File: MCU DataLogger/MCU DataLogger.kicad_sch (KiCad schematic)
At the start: 25 parts, among them U1 24LC1025, U2 DS1337S_, U3 ATMEGA328P-AN, U4 24LC1025, Y1 32.768 KHz, Y2 16MHz

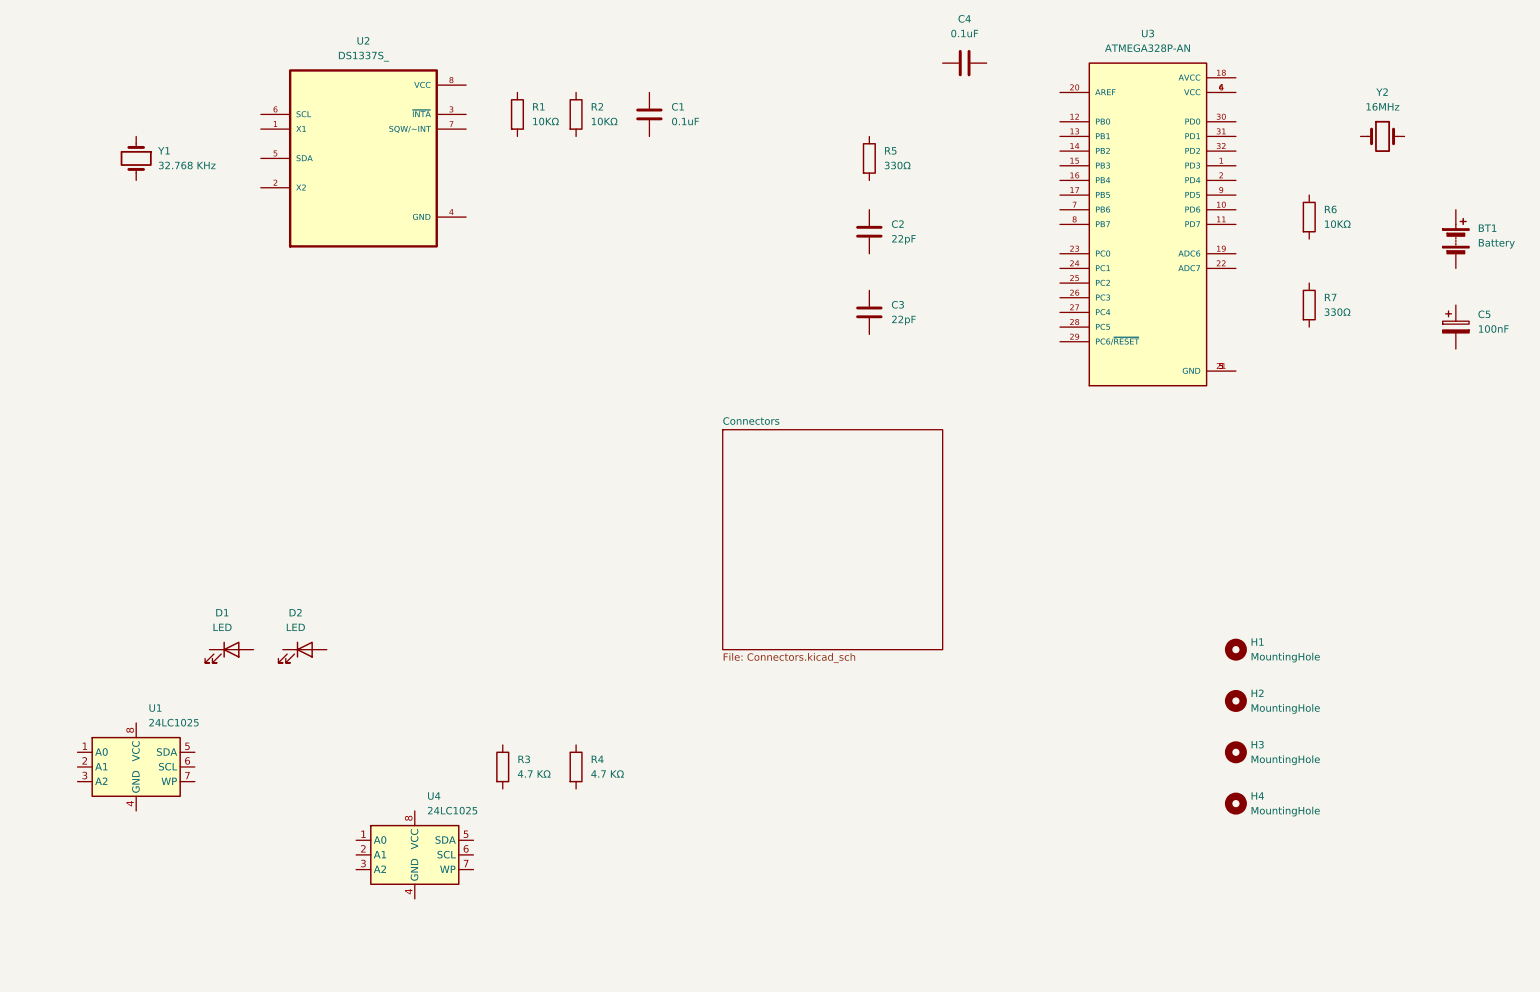
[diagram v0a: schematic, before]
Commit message: MCU Datalogger Project Schematic Complete
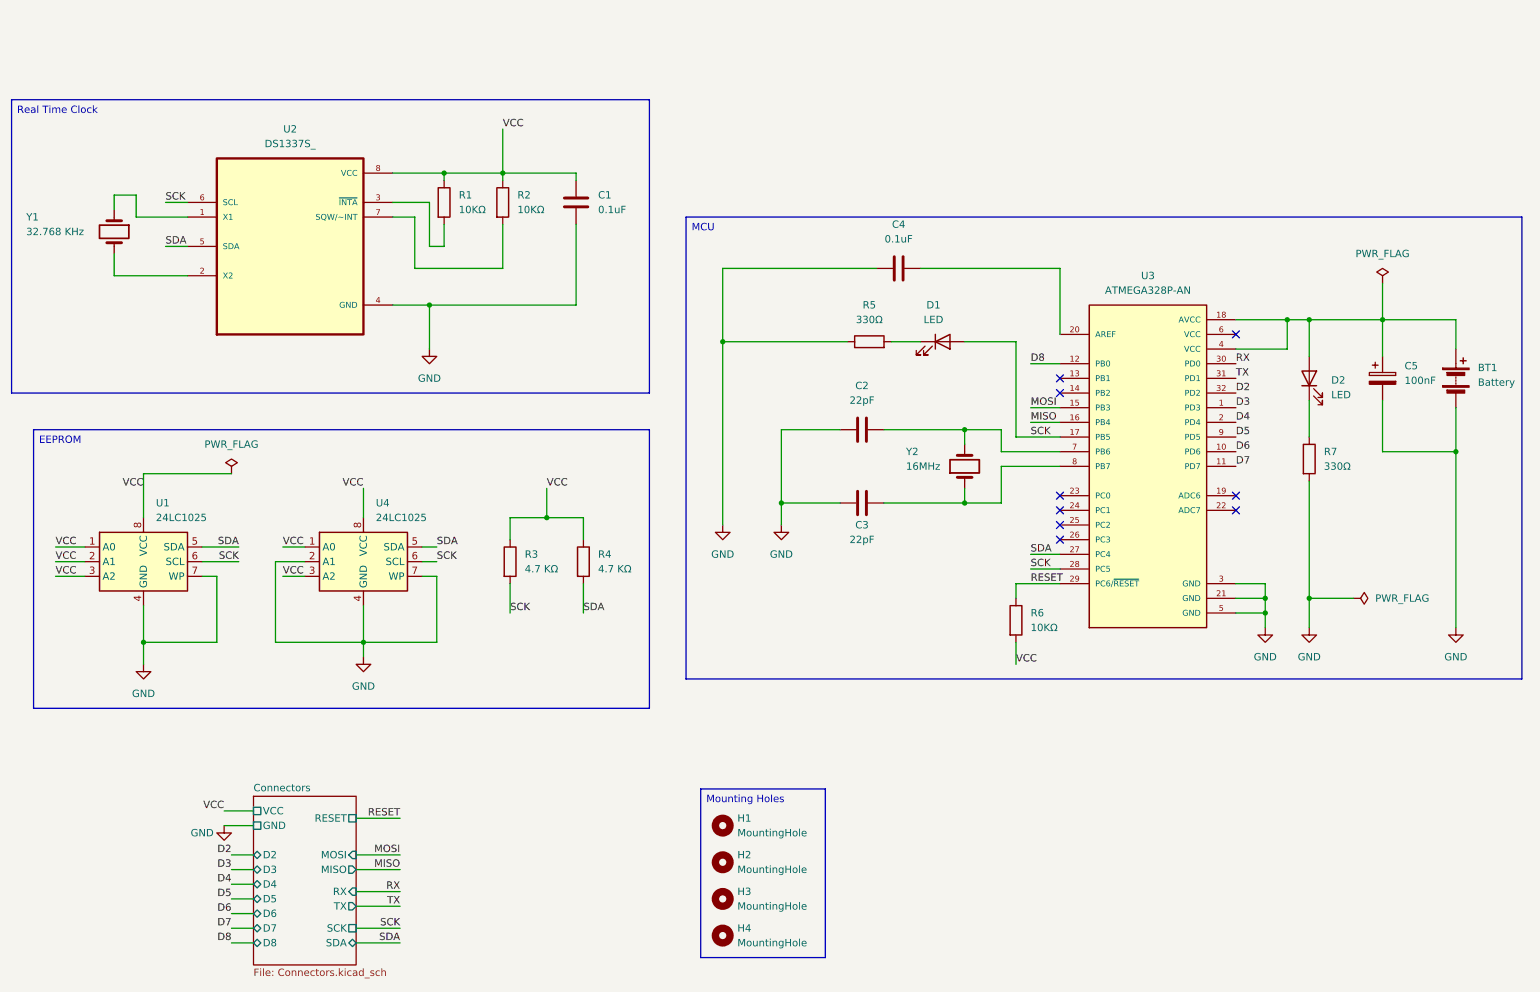
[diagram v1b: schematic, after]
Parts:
- U3: footprint ATMEGA328P:QFP80P900X900X120-32N -> ATMEGA328P-AN:QFP80P900X900X120-32N
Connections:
- net VCC: now reaches C1.1
- net VCC: now also R1.1, R2.1, R3.1, R4.1, R6.2, U1.1 (A0), U1.2 (A1), U1.3 (A2), U1.8 (VCC), U2.8 (VCC), U4.1 (A0), U4.3 (A2), U4.8 (VCC)
- net GND: now reaches C1.2
- net GND: now also BT1.2 (-), C2.1, C3.1, C4.1, C5.2, R5.1, R7.2, U1.4 (GND), U1.7 (WP), U2.4 (GND), U3.21 (GND), U3.3 (GND), U3.5 (GND), U4.2 (A1), U4.4 (GND), U4.7 (WP)
- net D3: now reaches U3.1 (PD3)
- net D6: now reaches U3.10 (PD6)
- net D7: now reaches U3.11 (PD7)
- net D8: now reaches U3.12 (PB0)
- net MOSI: now reaches U3.15 (PB3)
- net MISO: now reaches U3.16 (PB4)
- net SCK: now reaches U3.17 (PB5)
- net SCK: now also D1.2 (A), R3.2, U1.6 (SCL), U2.6 (SCL), U3.28 (PC5), U4.6 (SCL)
- net at U3.18 (AVCC): now also BT1.1 (+), C5.1, D2.2 (A), U3.4 (VCC)
- net D4: now reaches U3.2 (PD4)
- net at U3.20 (AREF): now also C4.2
- net SDA: now reaches U3.27 (PC4)
- net SDA: now also R4.2, U1.5 (SDA), U2.5 (SDA), U4.5 (SDA)
- net RESET: now reaches U3.29 (PC6/~{RESET})
- net RESET: now also R6.1
- net RX: now reaches U3.30 (PD0)
- net TX: now reaches U3.31 (PD1)
- net D2: now reaches U3.32 (PD2)
- net at U3.6 (VCC): no longer U3.4 (VCC)
- net at U3.7 (PB6): now also C2.2, Y2.2
- net at U3.8 (PB7): now also C3.2, Y2.1
- net D5: now reaches U3.9 (PD5)
- net at D2.1 (K): now also R7.1
- net at U2.1 (X1): now also Y1.1
- net at U2.2 (X2): now also Y1.2
- net at U2.3 (~{INTA}): now also R1.2
- net at U2.7 (SQW/~INT): now also R2.2
- net at D1.1 (K): now also R5.2
- no-connect marks 0 -> 9
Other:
- sheet Connectors ports: added D2, D3, D4, D5, D6, D7, D8, GND, MISO, MOSI, RESET, RX, SCK, SDA, TX, VCC; removed none
- moved on the sheet: BT1, C1, C2, C3, C4, C5, D1, D2, H1, H2, H3, H4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
